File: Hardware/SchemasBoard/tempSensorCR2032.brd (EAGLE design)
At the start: 26.2 x 13.4 mm, 16 parts, among them IC1 DS1820, T1 BC846, T2 BC846

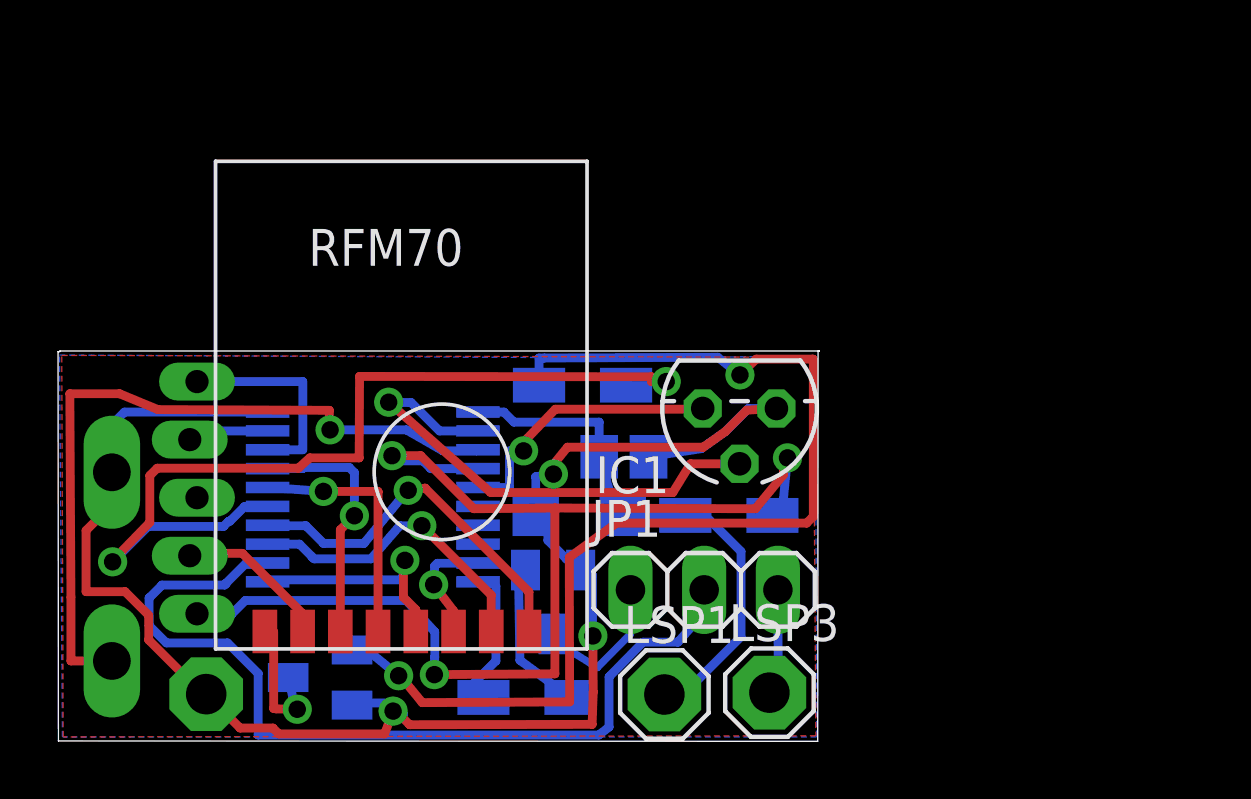
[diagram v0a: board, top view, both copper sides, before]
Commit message: aa
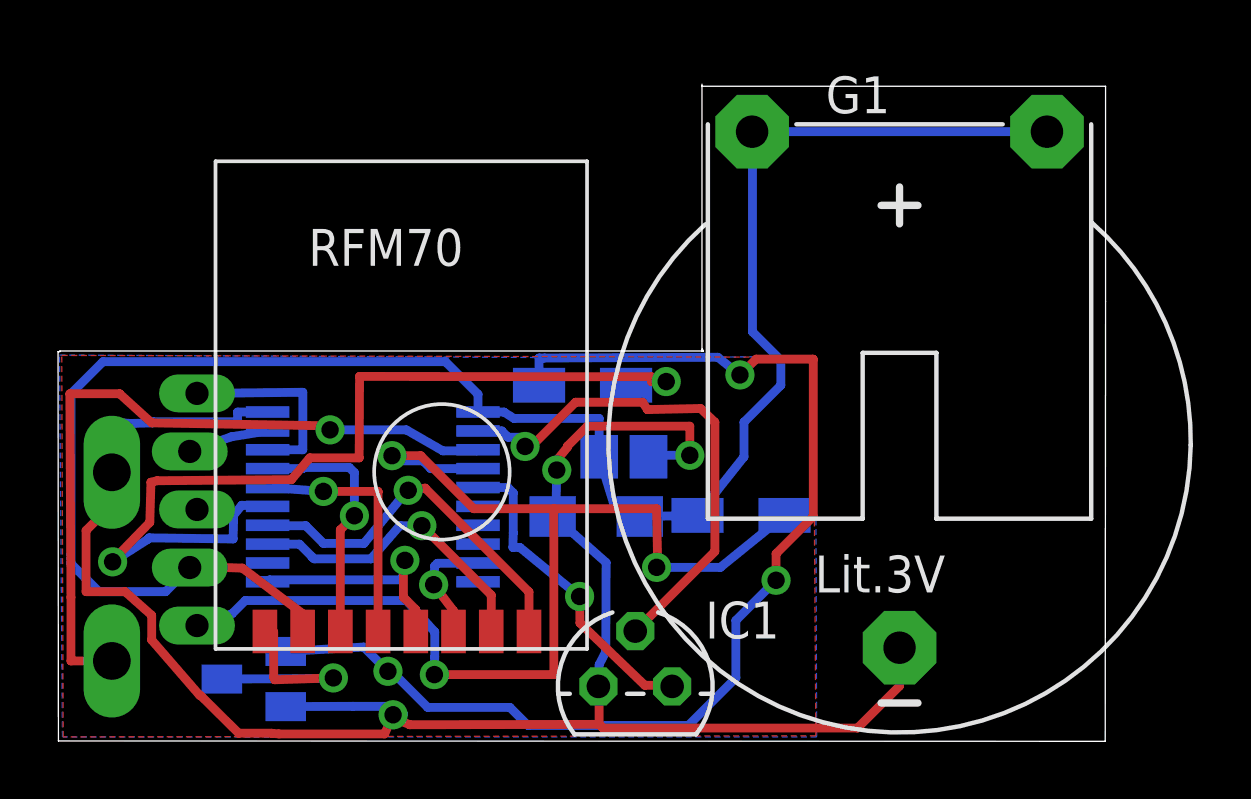
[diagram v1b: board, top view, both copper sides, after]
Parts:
- removed JP1: (no value), pinhead:1X03
- removed LSP1, LSP2, LSP3: SE14, solpad:SE14
- removed R2: 1K, resistor:R1206W
- removed T1: BC846, transistor:SOT23
- added G1: CR2032H, battery:CR2032H
- moved IC1 10.2 mm to (19.9, 1.88), turned to 0 degrees
- moved T2 2.29 mm to (6.73, 2.13)
- moved C2 0.58 mm to (18.5, 7.73)
- moved R1 0.42 mm to (23.5, 7.77)
- moved U$3 0.41 mm to (4.78, 7.98)
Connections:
- removed net N$4: JP1.2, U$2.12
- removed net N$5: JP1.3, LSP3.MP
- removed net N$6: R2.2, U$2.10
- removed net N$7: R2.1, T1.1
- removed net N$9: JP1.1, T1.3
- net GND: now also G1.-; no longer LSP2.MP, T1.2
- net VDD: now also G1.+; no longer LSP1.MP
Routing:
- net VDD: track 24.1 -> 66.4 mm
- net N$4: track 31.0 -> 0.00 mm
- net GND: track 59.3 -> 67.4 mm
- net N$9: track 6.12 -> 0.00 mm
- net N$7: track 5.51 -> 0.00 mm
- net N$6: track 4.98 -> 0.00 mm
- net N$5: track 3.74 -> 0.00 mm
- net N$13: track 4.91 -> 7.83 mm
- net N$14: track 38.4 -> 40.2 mm, vias 2 -> 3
- net N$3: track 9.75 -> 11.0 mm
- net N$1: track 17.3 -> 17.8 mm
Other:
- board size 26.2 x 13.4 mm -> 36.1 x 22.6 mm
